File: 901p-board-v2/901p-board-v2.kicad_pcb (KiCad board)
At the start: 2 copper layers, 32 parts, among them J1 USB-C (14 pins), J2 DE15, J3 AO(+/-), Q1 PMOS, U1 HUSB238_xxxDD, U3 ESP32-S3-DevKitC, U4 MAX3232, U5 NHD-C0220BIZ, U6 TPS63060

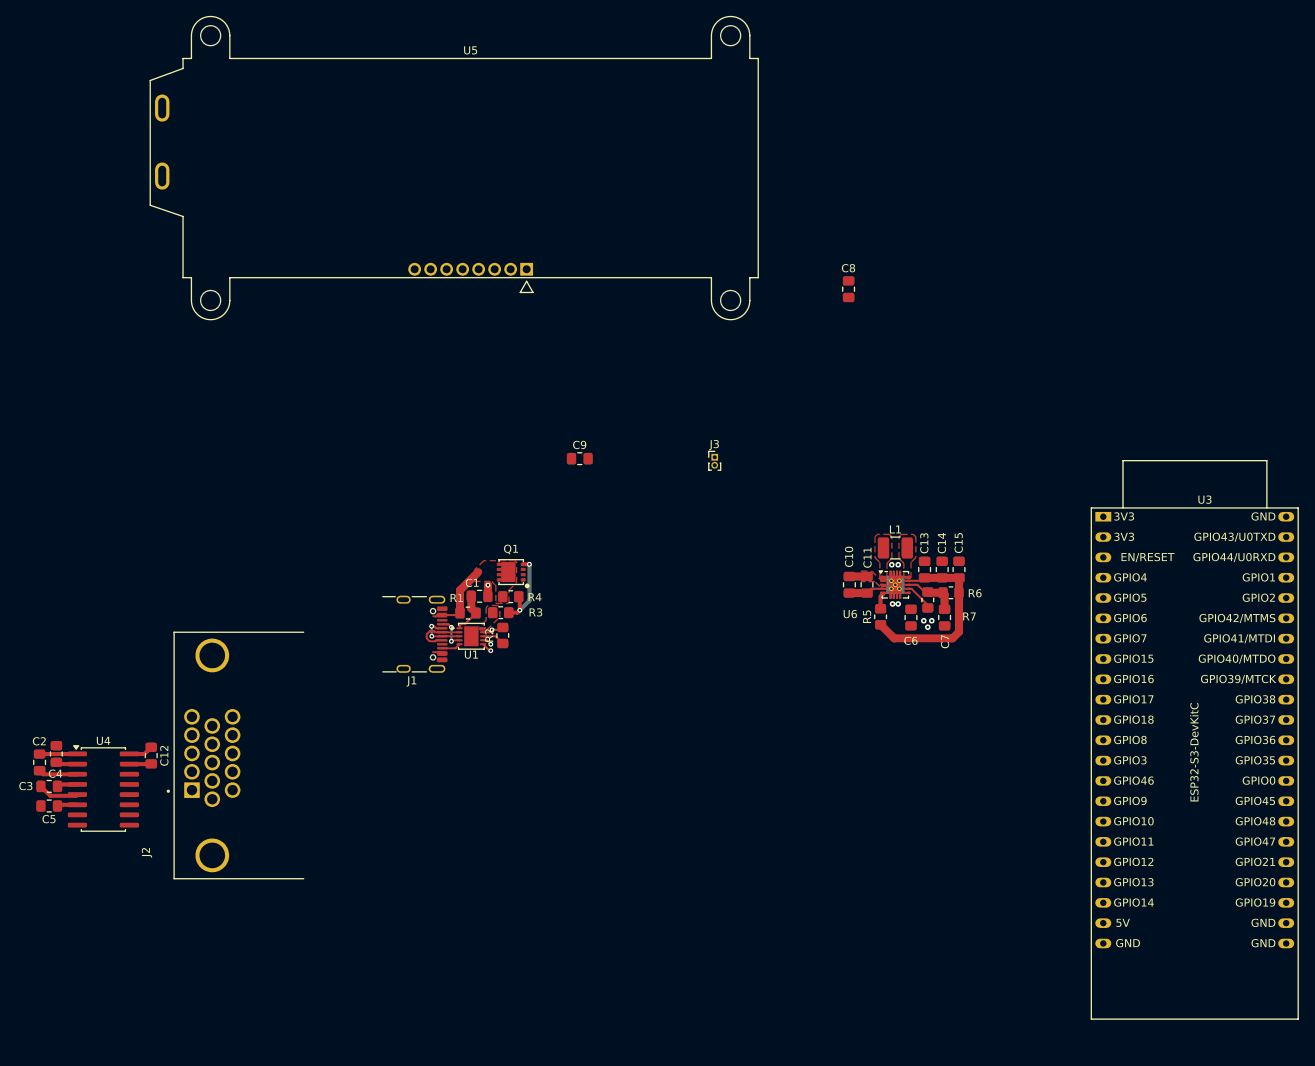
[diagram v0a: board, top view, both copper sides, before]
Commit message: finish v2 board
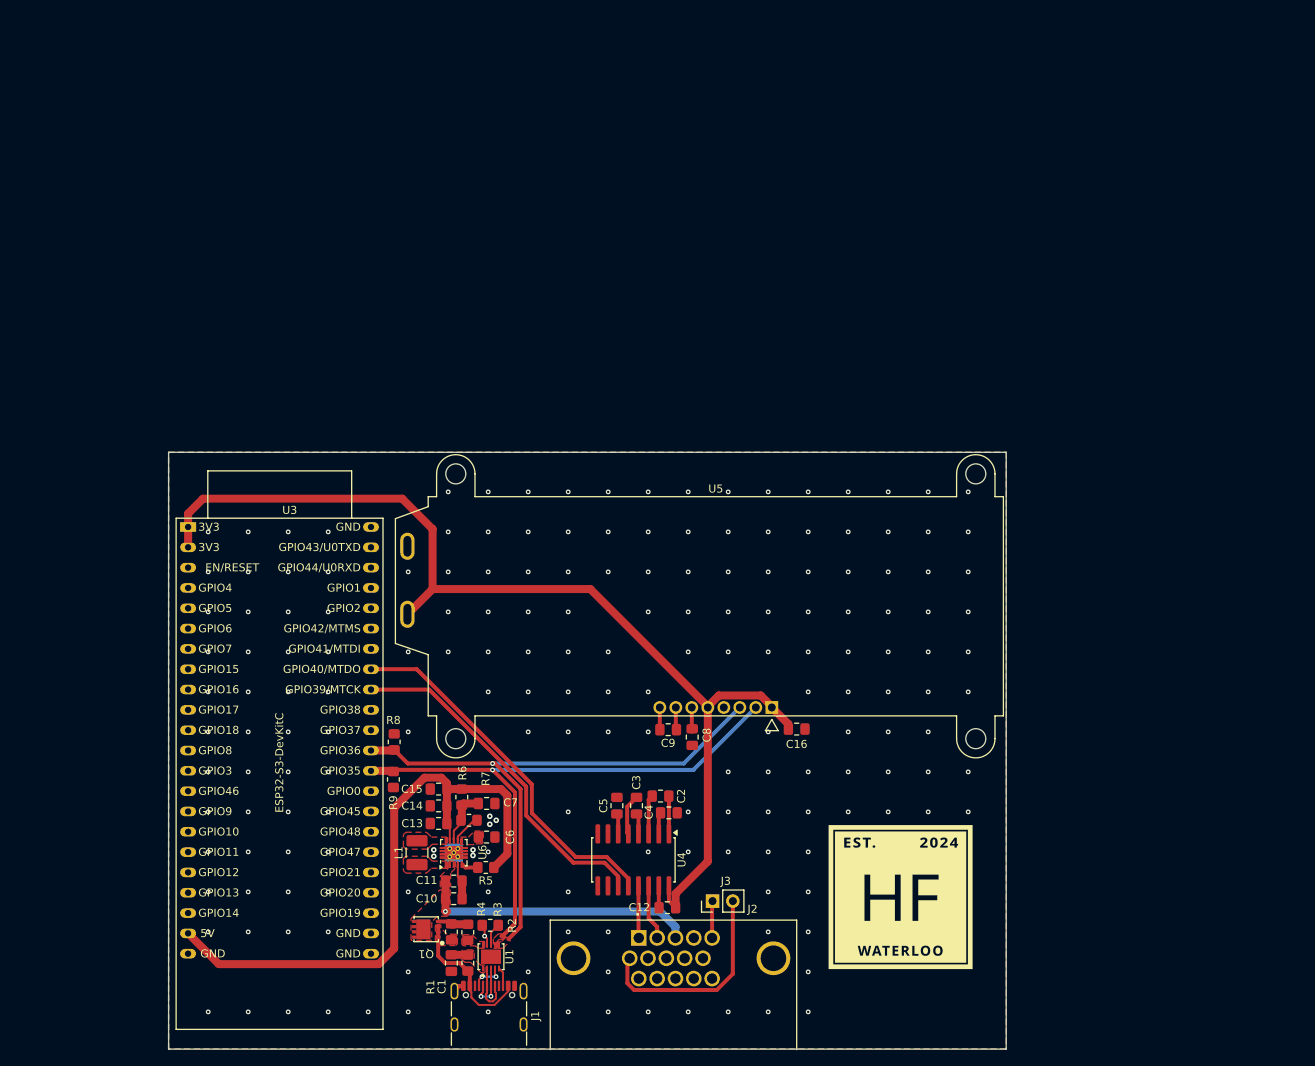
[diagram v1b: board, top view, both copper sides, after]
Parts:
- added C16: 100nF, Capacitor_SMD:C_0805_2012Metric_Pad1.18x1.45mm_HandSolder, F.Cu at (123.6, 104.3)
- added G***: LOGO, footprints:HF_logo, F.Cu at (136.6, 125.3)
- added R8: 5.1kΩ, Resistor_SMD:R_0805_2012Metric_Pad1.20x1.40mm_HandSolder, F.Cu at (73.3, 105.9)
- added R9: 5.1kΩ, Resistor_SMD:R_0805_2012Metric_Pad1.20x1.40mm_HandSolder, F.Cu at (73.2, 110.6)
- J3: footprint Connector_PinHeader_1.00mm:PinHeader_1x02_P1.00mm_Vertical -> Connector_PinHeader_2.54mm:PinHeader_1x02_P2.54mm_Vertical
- moved U3 114.4 mm to (47.5, 79.0)
- moved C2 77.7 mm to (106.6, 112.7), turned to 180 degrees
- moved C4 76.9 mm to (107.6, 114.8), turned to 0 degrees
- moved C3 73.5 mm to (103.6, 113.9), turned to 90 degrees
- moved C5 71.0 mm to (101.1, 113.9), turned to 90 degrees
- moved L1 70.9 mm to (76.2, 119.8), turned to 90 degrees
- moved C15 70.6 mm to (78.8, 111.8), turned to 180 degrees
- moved C14 69.5 mm to (78.8, 113.9), turned to 180 degrees
- moved C13 68.5 mm to (78.8, 116.1), turned to 180 degrees
- moved C12 67.3 mm to (107.4, 126.6), turned to 180 degrees
- moved U4 66.8 mm to (103.2, 120.7), turned to -90 degrees
- moved R6 66.3 mm to (81.8, 112.8), turned to -90 degrees
- moved U6 64.6 mm to (80.8, 119.8), turned to 90 degrees
- moved R7 63.6 mm to (82.7, 115.7), turned to 0 degrees
- moved C11 63.6 mm to (80.8, 123.3), turned to 0 degrees
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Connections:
- C8 pad 1: +3.3V -> Net-(U5-VOUT)
- C8 pad 2: Net-(U5-VOUT) -> GND
- J1 pad A4: Net-(Q1-D) -> Net-(Q1-S)
- J1 pad A9: Net-(Q1-D) -> Net-(Q1-S)
- J1 pad B4: Net-(Q1-D) -> Net-(Q1-S)
- J1 pad B9: Net-(Q1-D) -> Net-(Q1-S)
- Q1 pad 1: Net-(Q1-D) -> VBUS
- Q1 pad 3: VBUS -> Net-(Q1-S)
- R1 pad 1: Net-(Q1-D) -> Net-(Q1-S)
- R4 pad 2: Net-(Q1-D) -> Net-(Q1-S)
- U3 pad 32: unconnected-(U3-GPIO35-Pad32) -> /SCL
- U3 pad 33: unconnected-(U3-GPIO36-Pad33) -> /SDA
- U3 pad 36: unconnected-(U3-GPIO39/MTCK-Pad36) -> /SER_TX
- U3 pad 37: unconnected-(U3-GPIO40/MTDO-Pad37) -> /SER_RX
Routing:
- net +3.3V: track 3.07 -> 132.3 mm
- net /SCL: track 1.16 -> 74.2 mm
- net /SDA: track 1.28 -> 74.0 mm
- net +5V: track 24.2 -> 79.1 mm
- net /SER_RX: track 0.00 -> 46.0 mm
- net /SER_TX: track 0.00 -> 43.9 mm
- net VBUS: track 2.20 -> 34.7 mm, vias 0 -> 1
- net /AO-: track 0.00 -> 26.7 mm
- net Net-(Q1-S): track 0.00 -> 18.0 mm
- net Net-(Q1-D): track 10.8 -> 0.00 mm
- net Net-(U4-T1OUT): track 0.00 -> 6.95 mm
- net Net-(U4-R1IN): track 0.00 -> 6.53 mm
- net Net-(Q1-G): track 10.3 -> 3.84 mm, vias 2 -> 0
- net /AO+: track 0.00 -> 4.55 mm
- net Net-(U1-VIN): track 5.37 -> 2.07 mm
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- added copper zone on F.Cu, net /SCL
- added copper zone on F.Cu, net /SDA
- added copper zone on B.Cu, net GND
- added copper zone on F.Cu, net GND
- added copper zone on F.Cu, net Net-(Q1-S)
- added copper zone on F.Cu, net Net-(U1-VIN)
- added copper zone on F.Cu, net Net-(U6-VAUX)
- removed copper zone on F.Cu, net Net-(Q1-D)
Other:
- board outline added: 104.7 x 74.6 mm
